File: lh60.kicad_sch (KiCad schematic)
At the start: 26 parts

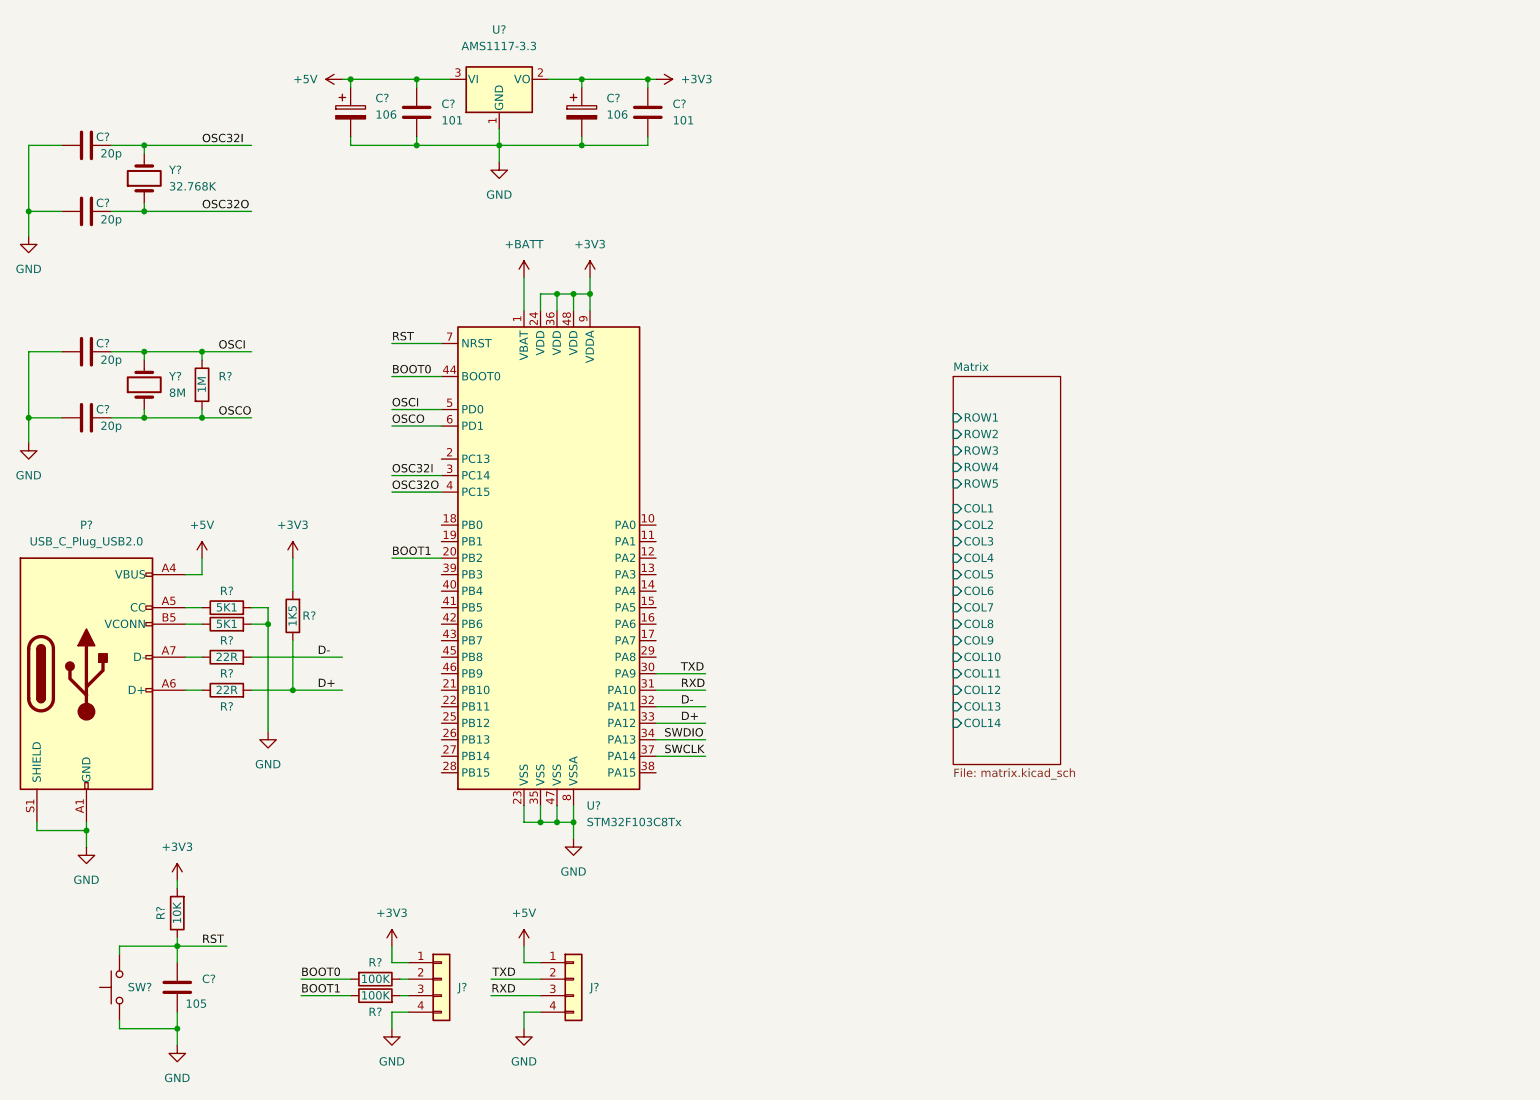
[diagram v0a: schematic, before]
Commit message: sch fin
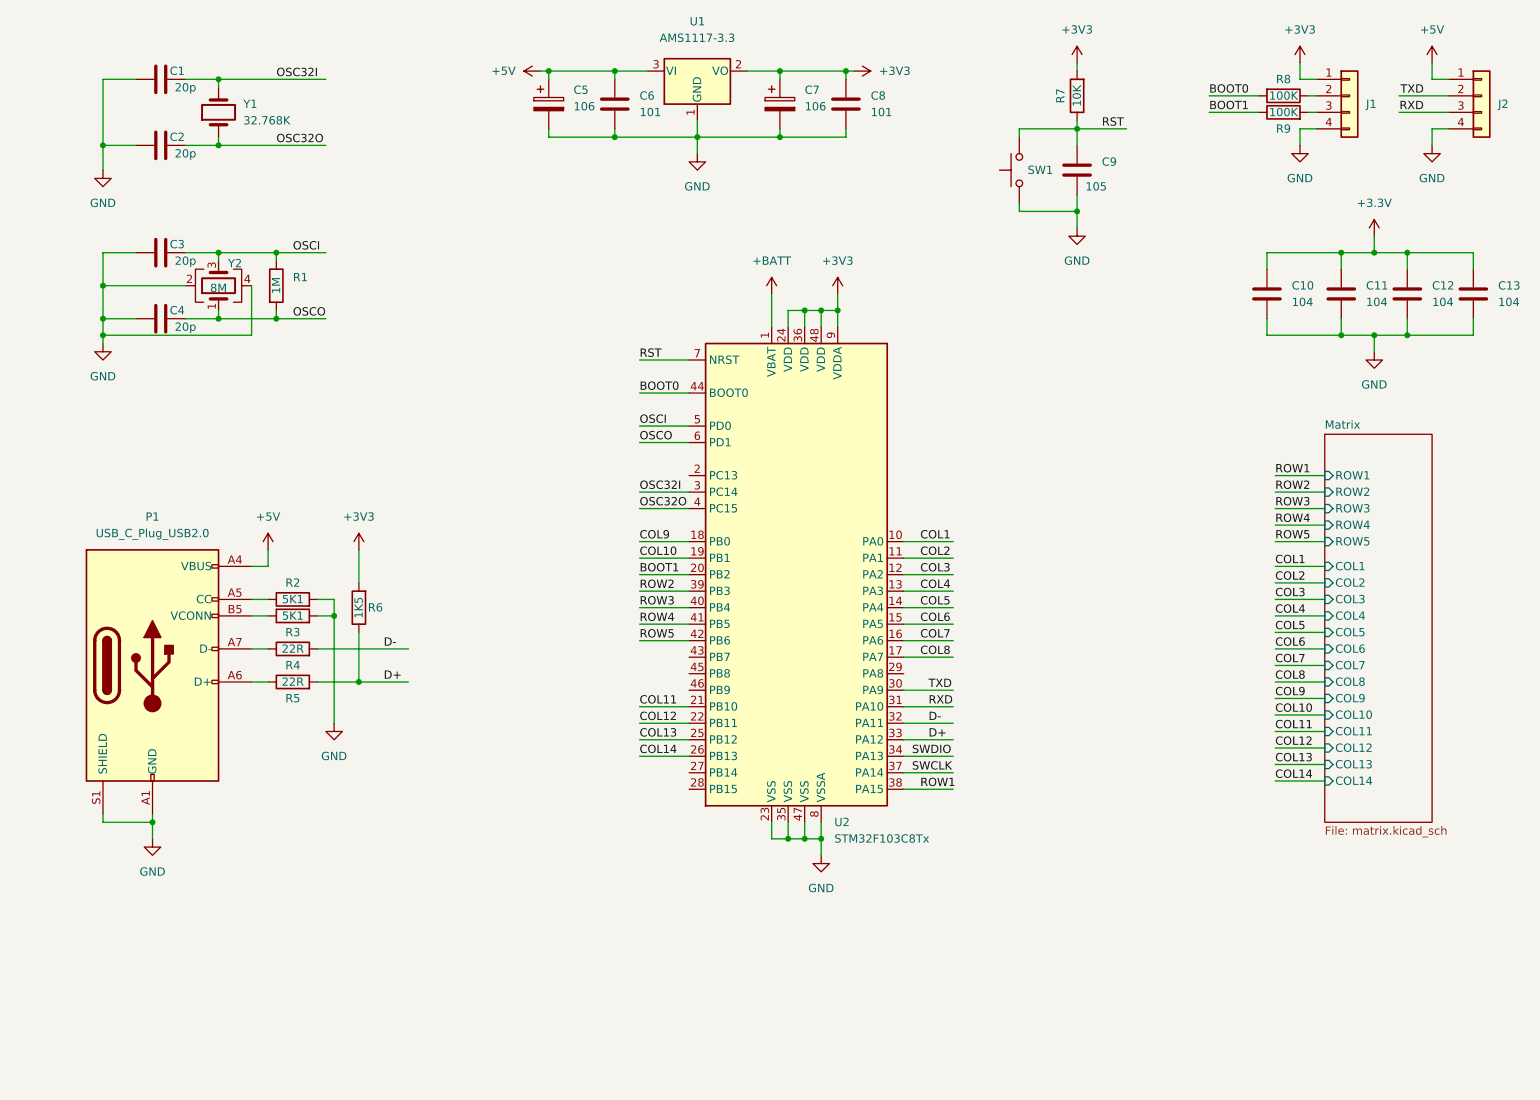
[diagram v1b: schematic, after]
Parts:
- removed Y?: 8M, symbol Device:Crystal
- added C10, C11, C12, C13: 104, Capacitor_SMD:C_0603_1608Metric_Pad1.08x0.95mm_HandSolder, symbol Device:C
- added Y2: 8M, Crystal:Crystal_SMD_3225-4Pin_3.2x2.5mm_HandSoldering, symbol Device:Crystal_GND24
- C1, C2, C3, C4, C5, C6, C7, C8, C9: renamed from C?; footprint (none) -> Capacitor_SMD:C_0603_1608Metric_Pad1.08x0.95mm_HandSolder
- J1, J2: renamed from J?; footprint (none) -> Connector_PinHeader_1.27mm:PinHeader_1x04_P1.27mm_Vertical
- P1: renamed from P?; footprint (none) -> Connector_USB:USB_C_Receptacle_HRO_TYPE-C-31-M-12
- R1, R2, R3, R4, R5, R6, R7, R8, R9: renamed from R?; footprint (none) -> Resistor_SMD:R_0603_1608Metric_Pad0.98x0.95mm_HandSolder
- SW1: renamed from SW?; footprint (none) -> Button_Switch_SMD:SW_SPST_FSMSM
- Y1: renamed from Y?; footprint (none) -> Crystal:Crystal_SMD_3215-2Pin_3.2x1.5mm
- gave numbers to parts that had none: 2
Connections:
- net +3V3: now also C10.1, C11.1, C12.1, C13.1
- net GND: now also C10.2, C11.2, C12.2, C13.2, Y2.2, Y2.4
- net OSCI: now also Y2.3
- net OSCO: now also Y2.1
- net COL1: now reaches U2.10 (PA0)
- net COL2: now reaches U2.11 (PA1)
- net COL3: now reaches U2.12 (PA2)
- net COL4: now reaches U2.13 (PA3)
- net COL5: now reaches U2.14 (PA4)
- net COL6: now reaches U2.15 (PA5)
- net COL7: now reaches U2.16 (PA6)
- net COL8: now reaches U2.17 (PA7)
- net COL9: now reaches U2.18 (PB0)
- net COL10: now reaches U2.19 (PB1)
- net COL11: now reaches U2.21 (PB10)
- net COL12: now reaches U2.22 (PB11)
- net COL13: now reaches U2.25 (PB12)
- net COL14: now reaches U2.26 (PB13)
- net ROW1: now reaches U2.38 (PA15)
- net ROW2: now reaches U2.39 (PB3)
- net ROW3: now reaches U2.40 (PB4)
- net ROW4: now reaches U2.41 (PB5)
- net ROW5: now reaches U2.42 (PB6)
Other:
- moved on the sheet: C1, C2, C3, C4, C5, C6, C7, C8, C9, J1, J2, P1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

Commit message: 20220326 pcb init
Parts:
- C5, C7: footprint Capacitor_SMD:C_0603_1608Metric_Pad1.08x0.95mm_HandSolder -> Capacitor_SMD:C_1206_3216Metric_Pad1.33x1.80mm_HandSolder
